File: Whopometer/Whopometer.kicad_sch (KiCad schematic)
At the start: 12 parts, among them U1 H3LIS331DLTR, U2 STM32F103C8Tx

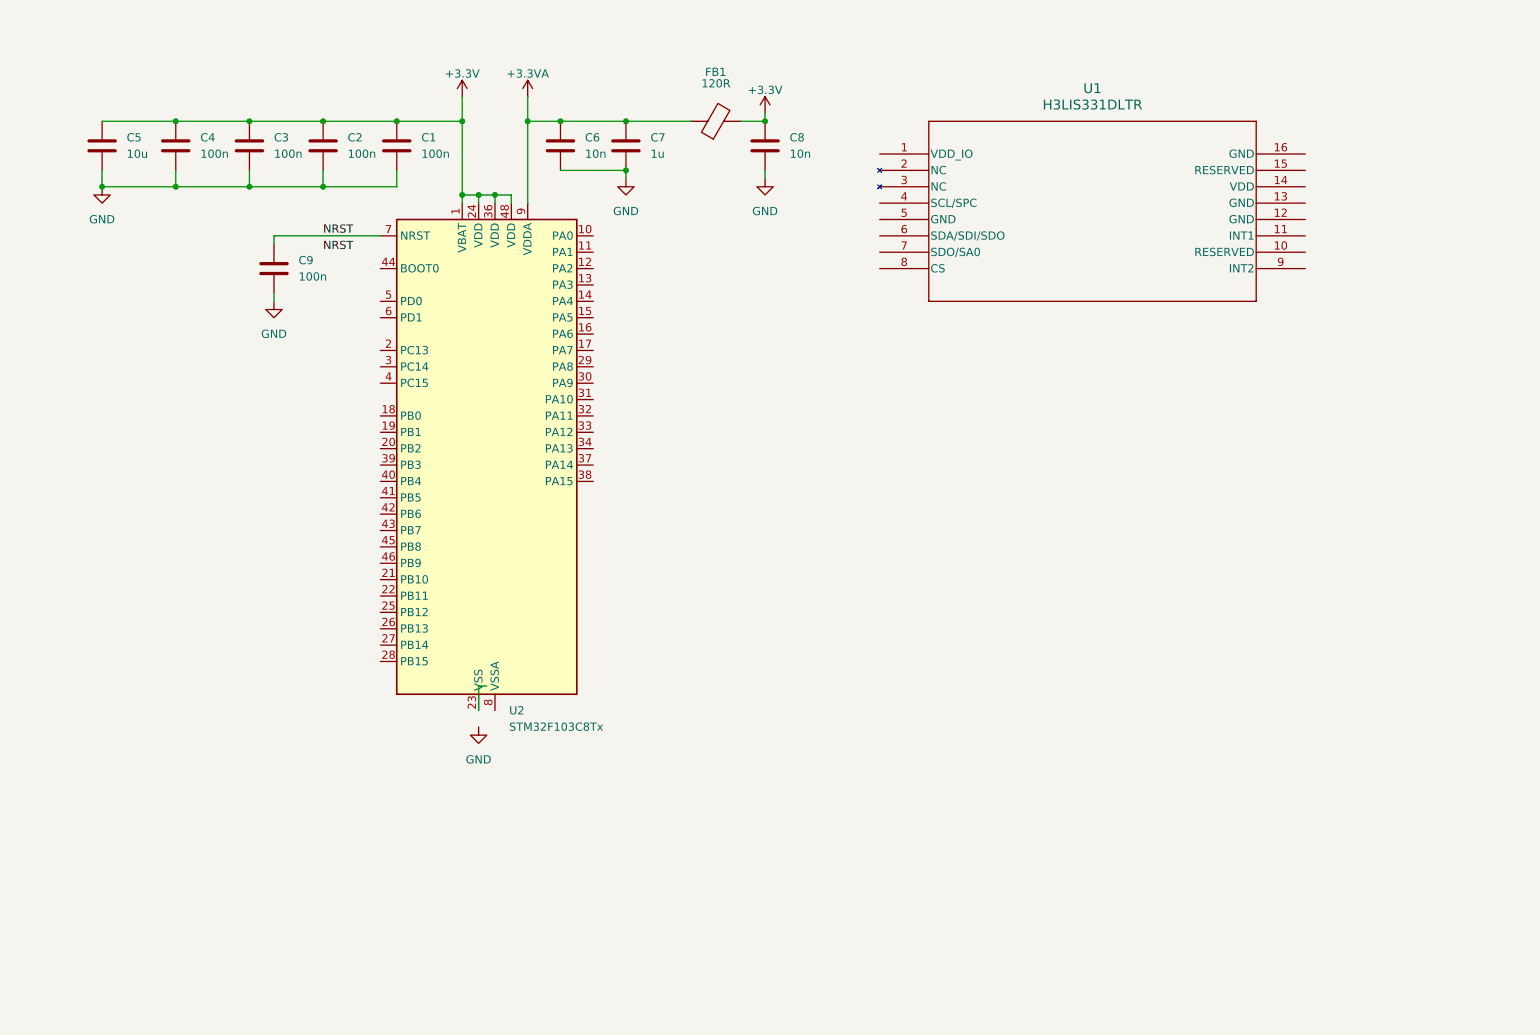
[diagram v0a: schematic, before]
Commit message: STM 32 time
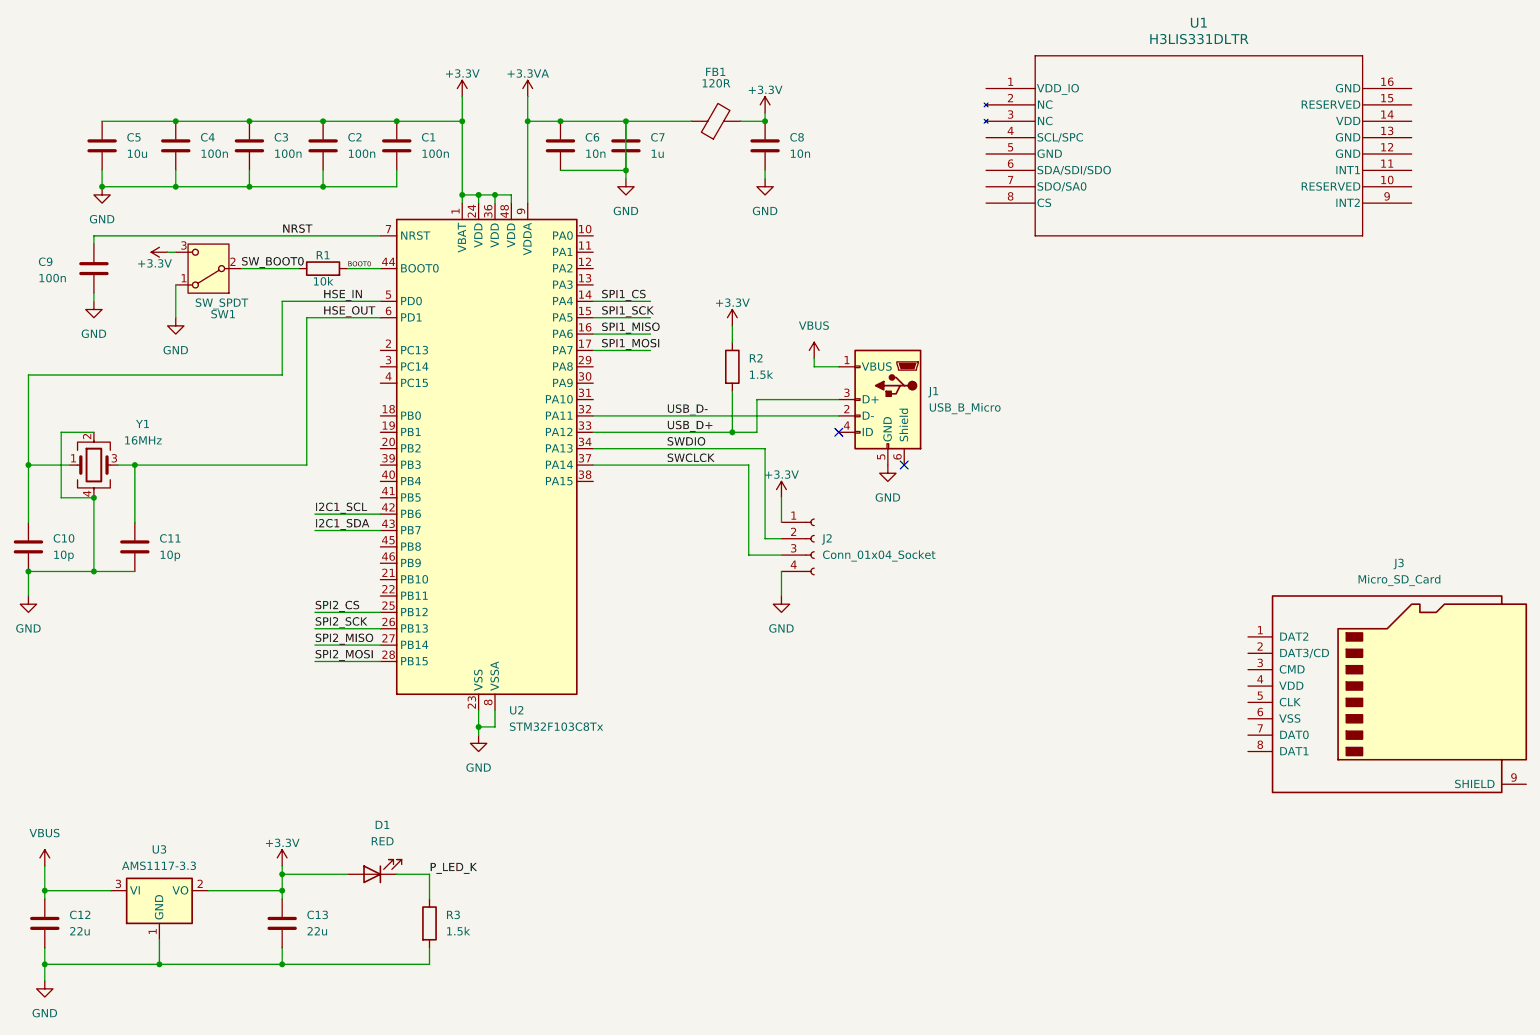
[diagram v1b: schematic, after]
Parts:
- added C10, C11: 10p, symbol Device:C
- added C12, C13: 22u, symbol Device:C
- added D1: RED, symbol Device:LED
- added J1: USB_B_Micro, symbol Connector:USB_B_Micro
- added J2: Conn_01x04_Socket, symbol Connector:Conn_01x04_Socket
- added J3: Micro_SD_Card, symbol Connector:Micro_SD_Card
- added R1: 10k, symbol Device:R
- added R2, R3: 1.5k, symbol Device:R
- added SW1: SW_SPDT, symbol Switch:SW_SPDT
- added U3: AMS1117-3.3, Package_TO_SOT_SMD:SOT-223-3_TabPin2, symbol Regulator_Linear:AMS1117-3.3
- added Y1: 16MHz, symbol Device:Crystal_GND24
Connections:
- net GND is gone; now on net +3.3VA: C1.2, C2.2, C3.2, C4.2, C5.2, C6.2, C7.2, C8.2, C9.2
- net +3.3V: now also C13.1, D1.2 (A), J2.1 (Pin_1), R2.1, SW1.3 (C), U3.2 (VO)
- net +3.3VA: now also U2.23 (VSS), U2.35 (VSS), U2.47 (VSS), U2.8 (VSSA), C10.2, C11.2, C12.2, C13.2, J1.5 (GND), J2.4 (Pin_4), R3.2, SW1.1 (A), U3.1 (GND), Y1.2, Y1.4
- net SPI1_CS: now reaches U2.14 (PA4)
- net SPI1_SCK: now reaches U2.15 (PA5)
- net SPI1_MISO: now reaches U2.16 (PA6)
- net SPI1_MOSI: now reaches U2.17 (PA7)
- net SPI2_CS: now reaches U2.25 (PB12)
- net SPI2_SCK: now reaches U2.26 (PB13)
- net SPI2_MISO: now reaches U2.27 (PB14)
- net SPI2_MOSI: now reaches U2.28 (PB15)
- net USB_D-: now reaches U2.32 (PA11)
- net USB_D-: now also J1.2 (D-)
- net USB_D+: now reaches U2.33 (PA12)
- net USB_D+: now also J1.3 (D+), R2.2
- net SWDIO: now reaches U2.34 (PA13)
- net SWDIO: now also J2.2 (Pin_2)
- net SWCLCK: now reaches U2.37 (PA14)
- net SWCLCK: now also J2.3 (Pin_3)
- net I2C1_SCL: now reaches U2.42 (PB6)
- net I2C1_SDA: now reaches U2.43 (PB7)
- net BOOT0: now reaches U2.44 (BOOT0)
- net BOOT0: now also R1.2
- net HSE_IN: now reaches U2.5 (PD0)
- net HSE_IN: now also C10.1, Y1.1
- net HSE_OUT: now reaches U2.6 (PD1)
- net HSE_OUT: now also C11.1, Y1.3
- new net P_LED_K: D1.1 (K), R3.1
- new net SW_BOOT0: R1.1, SW1.2 (B)
- new net VBUS: C12.1, J1.1 (VBUS), U3.3 (VI)
- no-connect marks 0 -> 2
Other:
- moved on the sheet: C9, U1
